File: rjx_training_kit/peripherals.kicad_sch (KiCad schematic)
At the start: 12 parts, among them J3 USB_OTG, SW3 SW_Push, U2 BME280, U3 DS3231M, U4 LTC-4627JD, U5 LIS3DH, U7 EMIF02-USB03F2

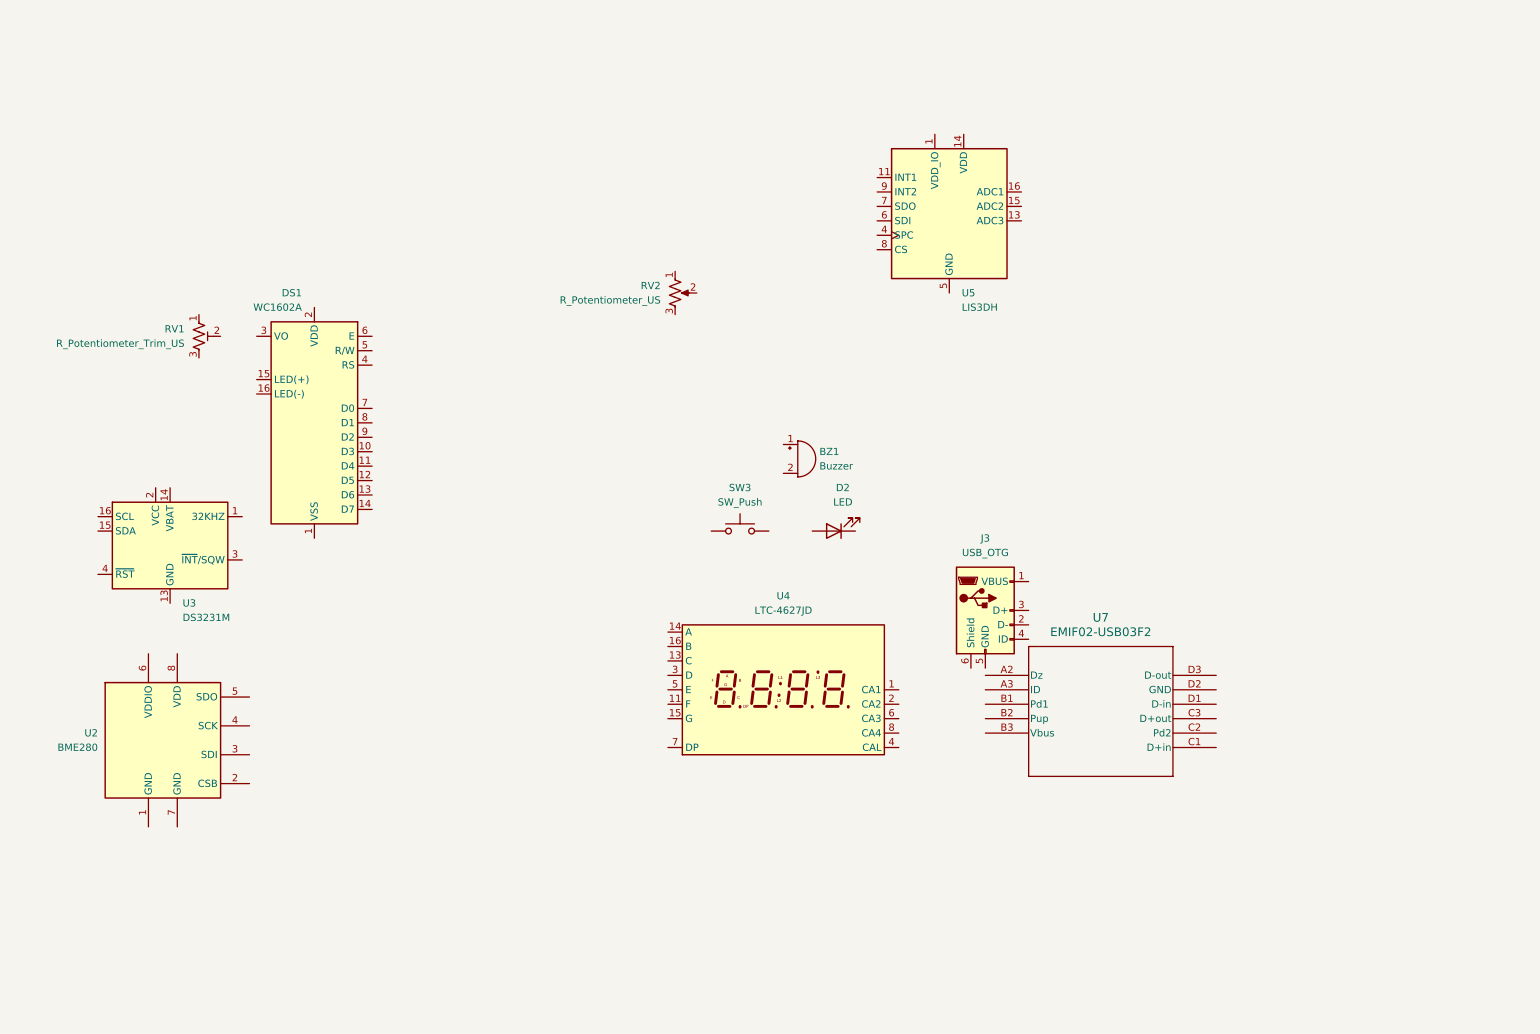
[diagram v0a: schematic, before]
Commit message: Update
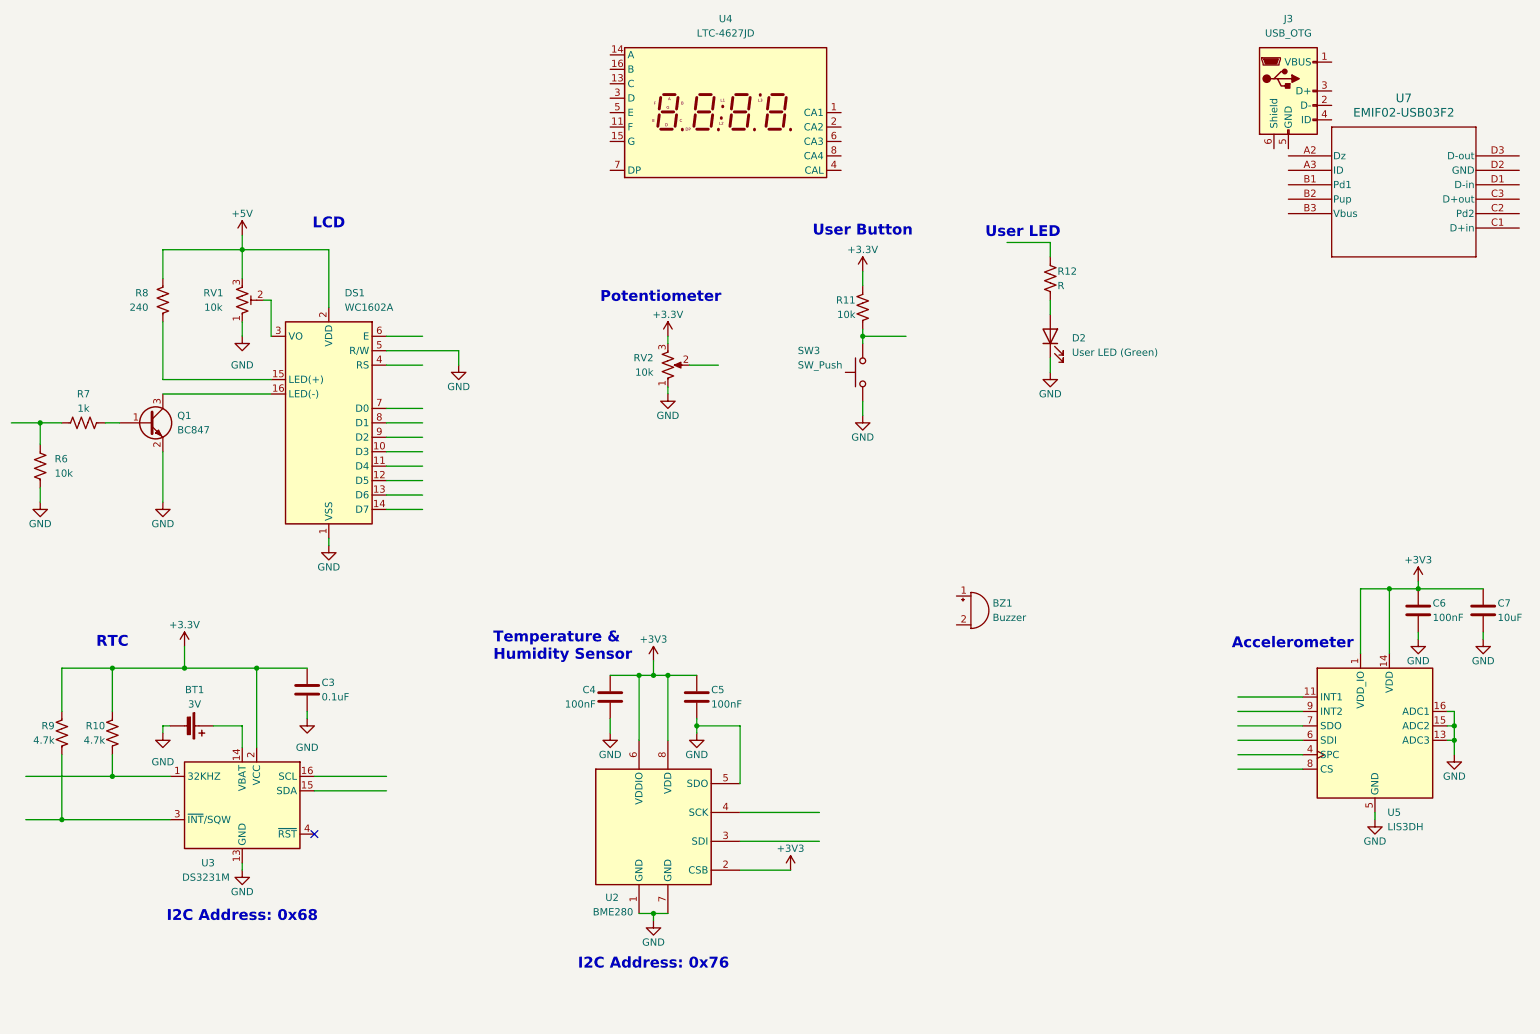
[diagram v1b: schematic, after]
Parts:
- added BT1: 3V, symbol Device:Battery_Cell
- added C3: 0.1uF, symbol Device:C
- added C4, C5, C6: 100nF, symbol Device:C
- added C7: 10uF, symbol Device:C
- added Q1: BC847, Package_TO_SOT_SMD:SOT-23, symbol Transistor_BJT:BC847
- added R10, R9: 4.7k, symbol Device:R_US
- added R11, R6: 10k, symbol Device:R_US
- added R12: R, symbol Device:R_US
- added R7: 1k, symbol Device:R_US
- added R8: 240, symbol Device:R_US
- D2: value LED -> User LED (Green)
- RV1: value R_Potentiometer_Trim_US -> 10k
- RV2: value R_Potentiometer_US -> 10k
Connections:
- net GND: now reaches RV1.1
- net GND: now also D2.1 (K), DS1.1 (VSS), DS1.5 (R/W), RV2.1, SW3.1, U2.1 (GND), U2.5 (SDO), U2.7 (GND), U3.10 (GND), U3.11 (GND), U3.12 (GND), U3.13 (GND), U3.5 (GND), U3.6 (GND), U3.7 (GND), U3.8 (GND), U3.9 (GND), U5.10 (GND), U5.12 (GND), U5.13 (ADC3), U5.15 (ADC2), U5.16 (ADC1), U5.5 (GND), BT1.2 (-), C3.2, C4.2, C5.2, C6.2, C7.2, Q1.2 (E), R6.2
- net at RV1.2: now also DS1.3 (VO)
- net +5V: now reaches RV1.3
- net +5V: now also DS1.2 (VDD), R8.2
- net at DS1.15 (LED(+)): now also R8.1
- net at DS1.16 (LED(-)): now also Q1.3 (C)
- net at U3.1 (32KHZ): now also R10.2
- net at U3.14 (VBAT): now also BT1.1 (+)
- net +3.3V: now reaches U3.2 (VCC)
- net +3.3V: now also RV2.3, C3.1, R10.1, R11.1, R9.1
- net at U3.3 (~{INT}/SQW): now also R9.2
- net at D2.2 (A): now also R12.2
- net +3V3: now reaches U5.1 (VDD_IO)
- net +3V3: now also U2.2 (CSB), U2.6 (VDDIO), U2.8 (VDD), U5.14 (VDD), C4.1, C5.1, C6.1, C7.1
- net at SW3.2: now also R11.2
- new net: Q1.1 (B), R7.2
- new net: R6.1, R7.1
- no-connect marks 0 -> 1
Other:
- note added: "Accelerometer"
- note added: "I2C Address: 0x68"
- note added: "I2C Address: 0x76"
- note added: "LCD"
- note added: "Potentiometer"
- note added: "RTC"
- note added: "Temperature & Humidity Sensor"
- note added: "User Button"
- note added: "User LED"
- moved on the sheet: BZ1, D2, DS1, J3, RV1, RV2, SW3, U2, U3, U4, U5, U7

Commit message: Update
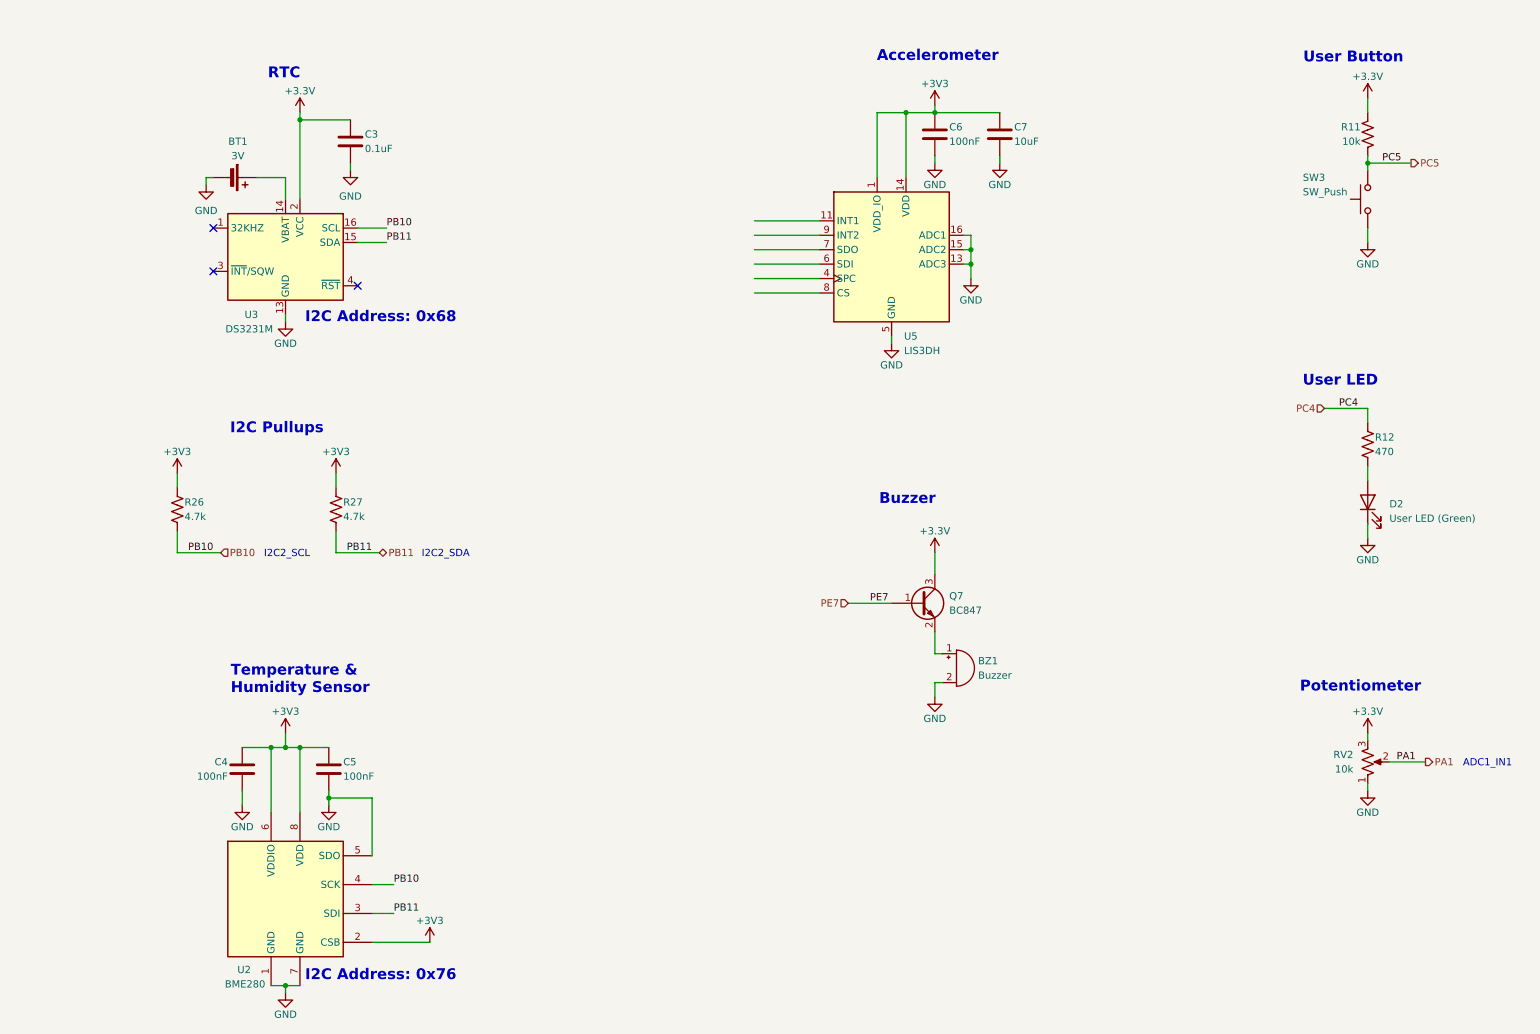
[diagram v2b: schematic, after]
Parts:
- removed DS1: WC1602A, Display:WC1602A, symbol Display_Character:WC1602A
- removed J3: USB_OTG, symbol Connector:USB_OTG
- removed Q1: BC847, Package_TO_SOT_SMD:SOT-23, symbol Transistor_BJT:BC847
- removed R10, R9: 4.7k, symbol Device:R_US
- removed R6: 10k, symbol Device:R_US
- removed R7: 1k, symbol Device:R_US
- removed R8: 240, symbol Device:R_US
- removed RV1: 10k, symbol Device:R_Potentiometer_Trim_US
- removed U4: LTC-4627JD, Display_7Segment:LTC-4627Jx, symbol Display_Character:LTC-4627JD
- removed U7: EMIF02-USB03F2, FLIP-CHIP11_1P44X1P94_STM, symbol emif02-usb03f2:EMIF02-USB03F2
- added Q7: BC847, Package_TO_SOT_SMD:SOT-23, symbol Transistor_BJT:BC847
- added R26, R27: 4.7k, symbol Device:R_US
- R12: value R -> 470
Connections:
- net +3.3V: now also Q7.3 (C)
- net +3V3: now also R26.1, R27.1
- net GND: now also BZ1.2 (-)
- net PC4: now reaches R12.1
- net PB11: now reaches U3.15 (SDA)
- net PB11: now also U2.3 (SDI), R27.2
- net PB10: now reaches U3.16 (SCL)
- net PB10: now also U2.4 (SCK), R26.2
- net at BZ1.1 (+): now also Q7.2 (E)
- net PC5: now reaches R11.2, SW3.2
- net PA1: now reaches RV2.2
- new net PE7: Q7.1 (B)
- no-connect marks 1 -> 3
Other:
- note added: "ADC1_IN1"
- note added: "Buzzer"
- note added: "I2C Pullups"
- note added: "I2C2_SCL"
- note added: "I2C2_SDA"
- note removed: "LCD"
- moved on the sheet: BT1, BZ1, C3, C4, C5, C6, C7, D2, R11, R12, RV2, SW3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
